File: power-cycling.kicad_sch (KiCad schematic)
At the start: 89 parts

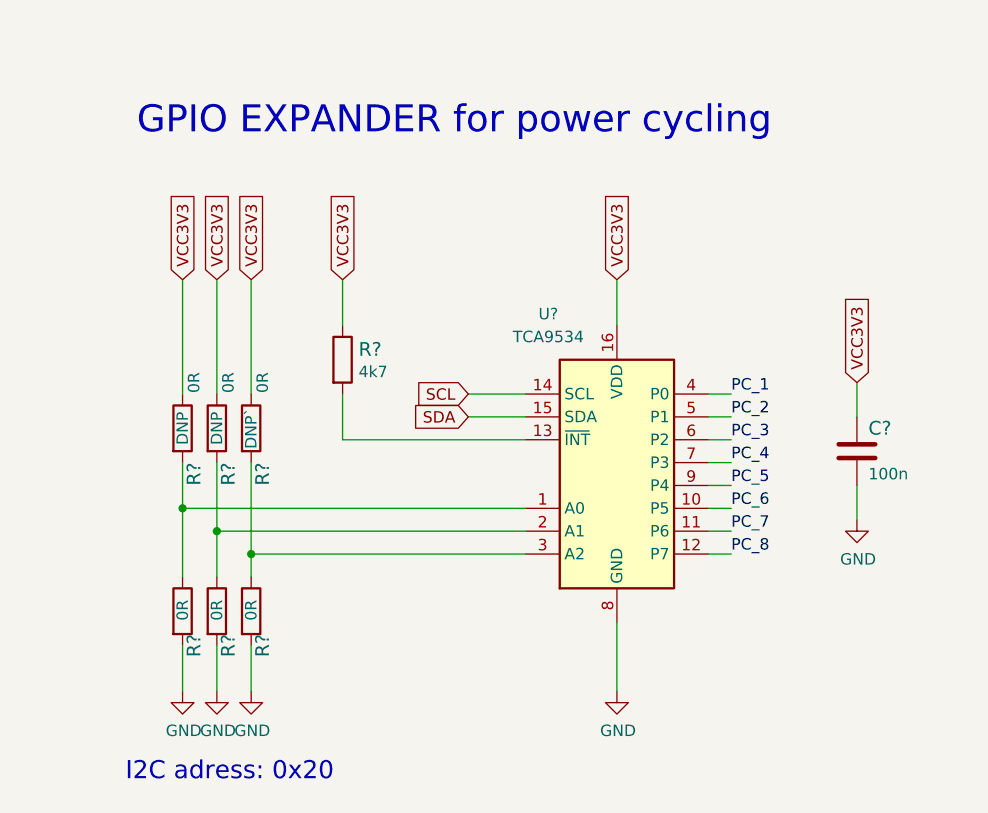
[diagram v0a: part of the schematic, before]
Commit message: WIP Standarization
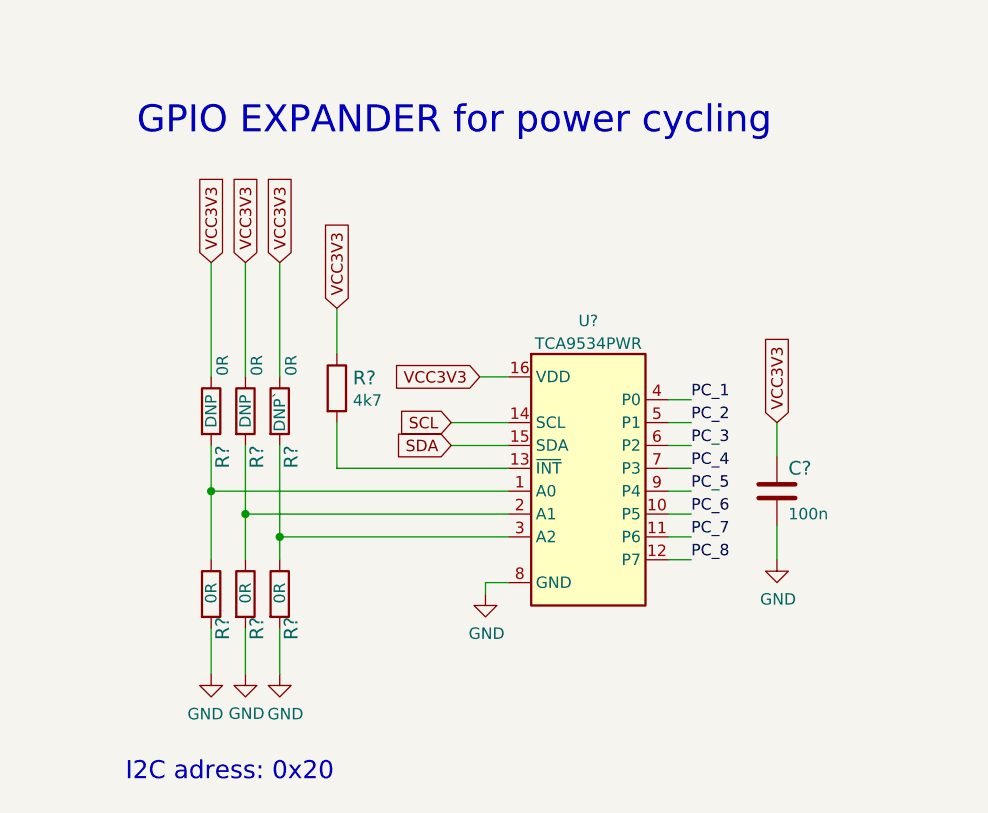
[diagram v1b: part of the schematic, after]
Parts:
- removed R? (x6): R_0R_0402, antmicro-footprints:R_0402_1005Metric, symbol antmicroResistors0402:R_0R_0402
- removed R?: R_4k7_0402, antmicro-footprints:R_0402_1005Metric, symbol antmicroResistors0402:R_4k7_0402
- removed U?: TCA9534, gpu-cluster-backplane-footprints:TSSOP-16, symbol gpu-cluster-backplane:TCA9534
- added R? (x6): R_0R_0402, antmicro-footprints:R_0402_1005Metric, symbol antmicroResistors0402:R_0R_0402
- added R?: R_4k7_0402, antmicro-footprints:R_0402_1005Metric, symbol antmicroResistors0402:R_4k7_0402
- added U?: TCA9534PWR, antmicro-footprints:TSSOP-16_4.4x5mm_P0.65mm, symbol antmicroInterfaceIOExpanders:TCA9534PWR
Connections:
- net GND: now also R?.2, R?.2, R?.2, U?.8 (GND)
- net PC_1: now also U?.4 (P0)
- net PC_2: now also U?.5 (P1)
- net PC_3: now also U?.6 (P2)
- net PC_4: now also U?.7 (P3)
- net PC_5: now also U?.9 (P4)
- net PC_6: now also U?.10 (P5)
- net PC_7: now also U?.11 (P6)
- net PC_8: now also U?.12 (P7)
- net SCL: now also U?.14 (SCL)
- net SDA: now also U?.15 (SDA)
- net VCC3V3: now also R?.1, R?.1, R?.1, R?.1, U?.16 (VDD)
- new net: R?.1, R?.2, U?.1 (A0)
- new net: R?.2, U?.13 (~{INT})
- new net: R?.1, R?.2, U?.2 (A1)
- new net: R?.1, R?.2, U?.3 (A2)
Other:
- moved on the sheet: C?
